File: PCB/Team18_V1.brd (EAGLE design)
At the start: 100 x 80 mm, 7 parts, among them IC1 STM32F746ZGT6

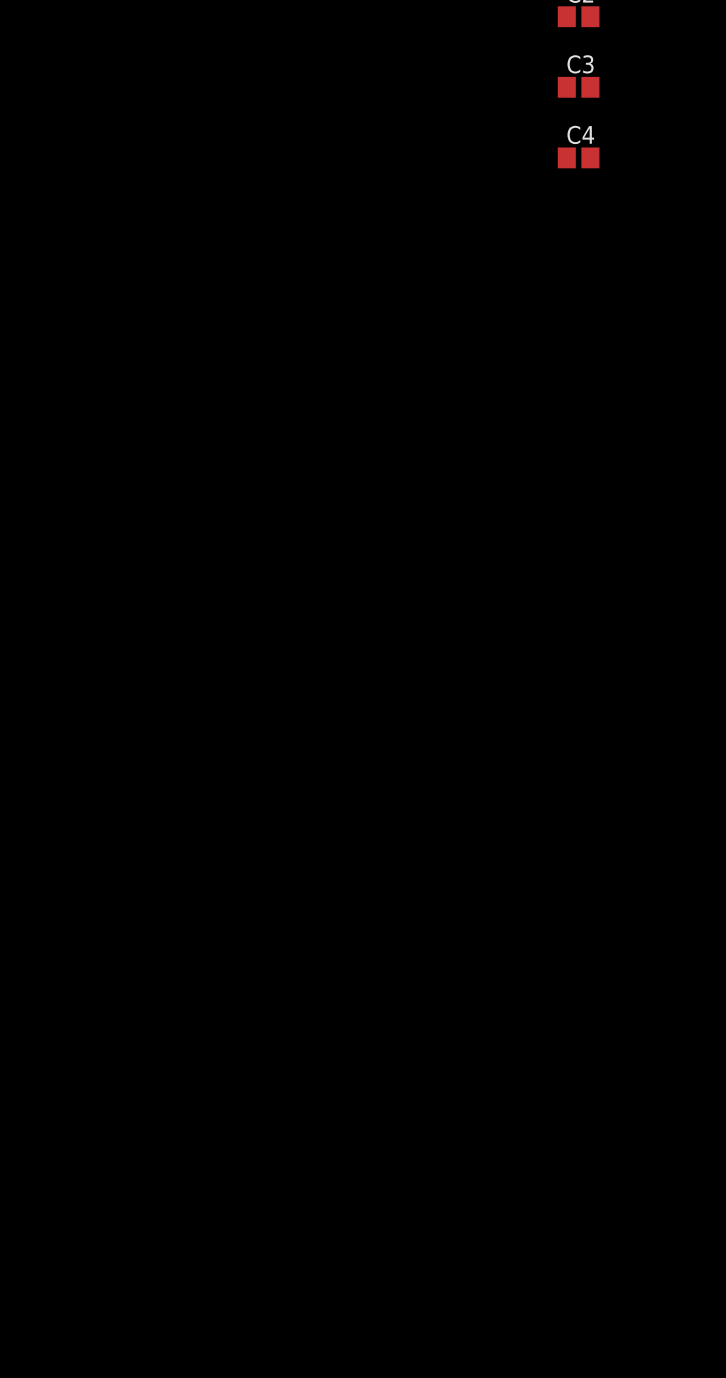
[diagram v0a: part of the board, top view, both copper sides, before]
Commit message: PCB
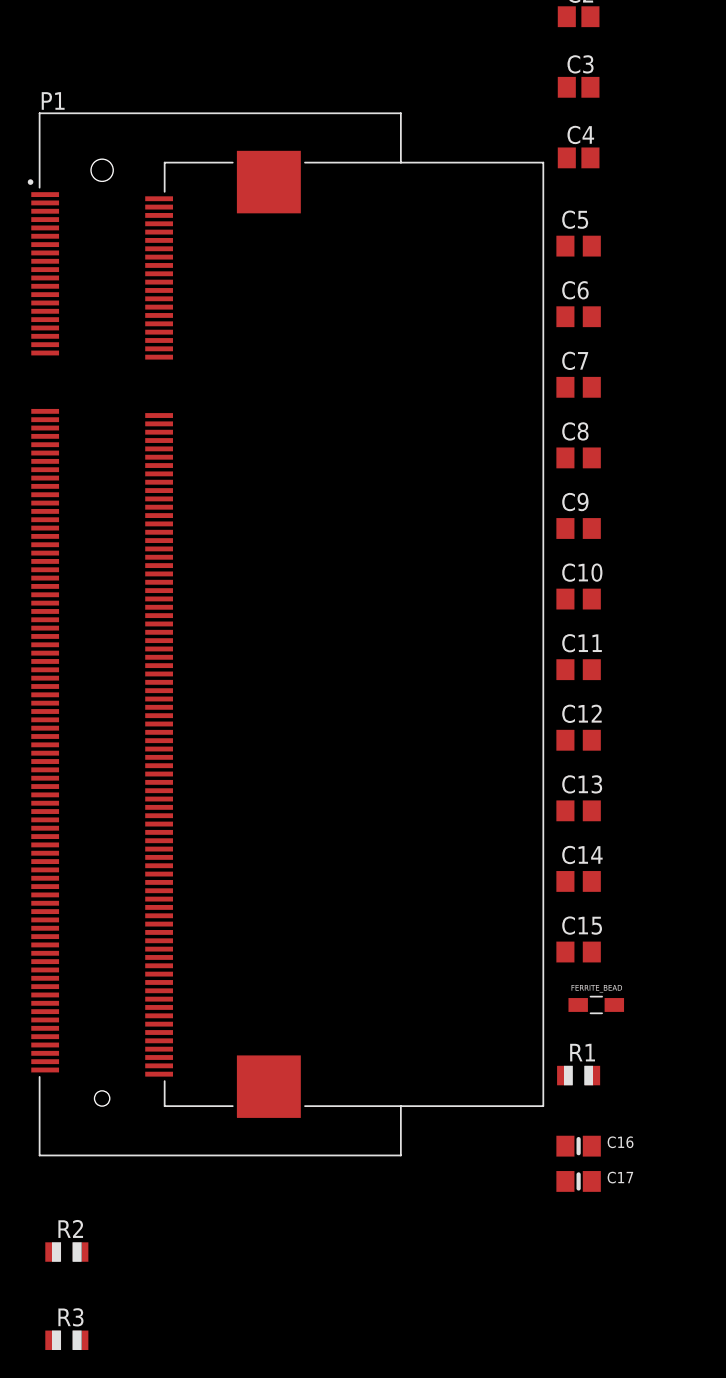
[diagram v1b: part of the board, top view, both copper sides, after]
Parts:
- added C10, C11, C12, C13, C14, C15, C5, C6, C7, C8: 100nF, rcl:C0805
- added C16, C17: 2.2uF, audio amplifier example:0805-NO
- added C9: (no value), rcl:C0805
- added FERRITE_BEAD: (no value), Wurth_Elektronik_Passive_rev18f:WE-CBA_0805(W=4)
- added P1: 1-1473005-4, Rpi-DDR2:TE_1-1473005-4
- added R1: 0, audio amplifier example:R0805
- added R2: 1k, audio amplifier example:R0805
- added R3: 10k, audio amplifier example:R0805
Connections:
- removed net N$3: C1.2
- removed net N$4: C2.2
- removed net VDD_1: IC1.17
- removed net VDD_10: IC1.131
- removed net VDD_11: IC1.144
- removed net VDD_2: IC1.30
- removed net VDD_3: IC1.39
- removed net VDD_4: IC1.52
- removed net VDD_5: IC1.62
- removed net VDD_6: IC1.72
- removed net VDD_7: IC1.84
- removed net VDD_8: IC1.108
- removed net VDD_9: IC1.121
- removed net VSSA: IC1.31
- removed net VSS_1: IC1.16
- removed net VSS_2: IC1.38
- removed net VSS_3: IC1.51
- removed net VSS_4: IC1.61
- removed net VSS_5: IC1.83
- removed net VSS_7: IC1.107
- removed net VSS_8: IC1.120
- removed net VSS_9: IC1.130
- new net 3.3V: P1.191, P1.192, P1.193, P1.194, R3.2
- new net GND: C1.2, C10.2, C11.2, C12.2, C13.2, C14.1, C15.1, C16.2, C17.2, C2.2, C3.2, C4.2, C5.1, C6.1, C7.1, C8.2, C9.2, HIGH_FREQ_OSC.2, HIGH_FREQ_OSC.4, IC1.107, IC1.120, IC1.130, IC1.16, IC1.31, IC1.38, IC1.51, IC1.61, IC1.83, P1.1, P1.103, P1.104, P1.109, P1.110, P1.115, P1.116, P1.121, P1.122, P1.127, P1.13, P1.133, P1.134, P1.139, P1.14, P1.140, P1.145, P1.146, P1.151, P1.152, P1.157, P1.163, P1.164, P1.169, P1.170, P1.181, P1.182, P1.187, P1.188, P1.19, P1.195, P1.196, P1.20, P1.25, P1.26, P1.31, P1.32, P1.37, P1.38, P1.43, P1.44, P1.49, P1.50, P1.55, P1.56, P1.61, P1.62, P1.67, P1.68, P1.7, P1.73, P1.74, P1.79, P1.8, P1.80, P1.85, P1.86, P1.91, P1.92, P1.97, P1.98, R2.2
- new net OSC32_IN: C1.1, IC1.8, LOW_FREQ_OSC.X1
- new net OSC32_OUT: C2.1, IC1.9, LOW_FREQ_OSC.X2
- new net OSC_IN: C3.1, HIGH_FREQ_OSC.1, IC1.23
- new net OSC_OUT: C4.1, HIGH_FREQ_OSC.3, IC1.24
- new net RUN: P1.177, R3.1
- new net USB_OTGID: P1.168, R2.1
- new net VBAT: P1.197, P1.198, P1.199, P1.200
- new net VBATSTM: IC1.5
- new net VDD: C10.1, C11.1, C12.1, C13.1, C14.2, C15.2, C5.2, C6.2, C7.2, C8.1, C9.1, FERRITE_BEAD.1, IC1.108, IC1.121, IC1.131, IC1.144, IC1.17, IC1.30, IC1.39, IC1.52, IC1.62, IC1.72, IC1.84
- new net VREF: IC1.32, R1.2
- net N$1: now also C16.1, IC1.71; no longer C1.1, LOW_FREQ_OSC.X1
- net N$2: now also C17.1, IC1.106; no longer C2.1, LOW_FREQ_OSC.X2
- net VDDA: now also FERRITE_BEAD.2, R1.1
